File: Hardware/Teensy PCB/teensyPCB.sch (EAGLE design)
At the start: 14 parts, among them U2 USD-SOCKETNEW

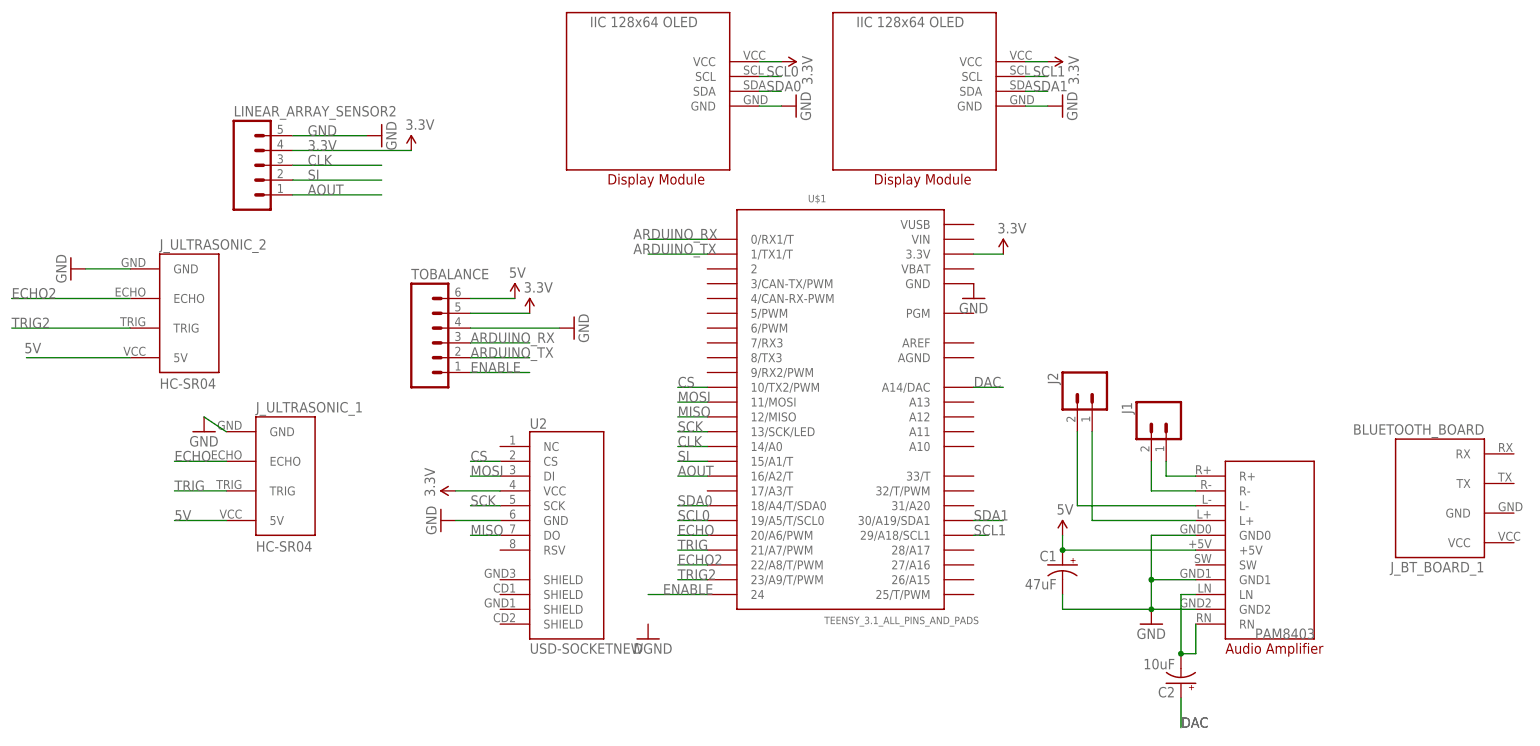
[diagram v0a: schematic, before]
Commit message: pcb update
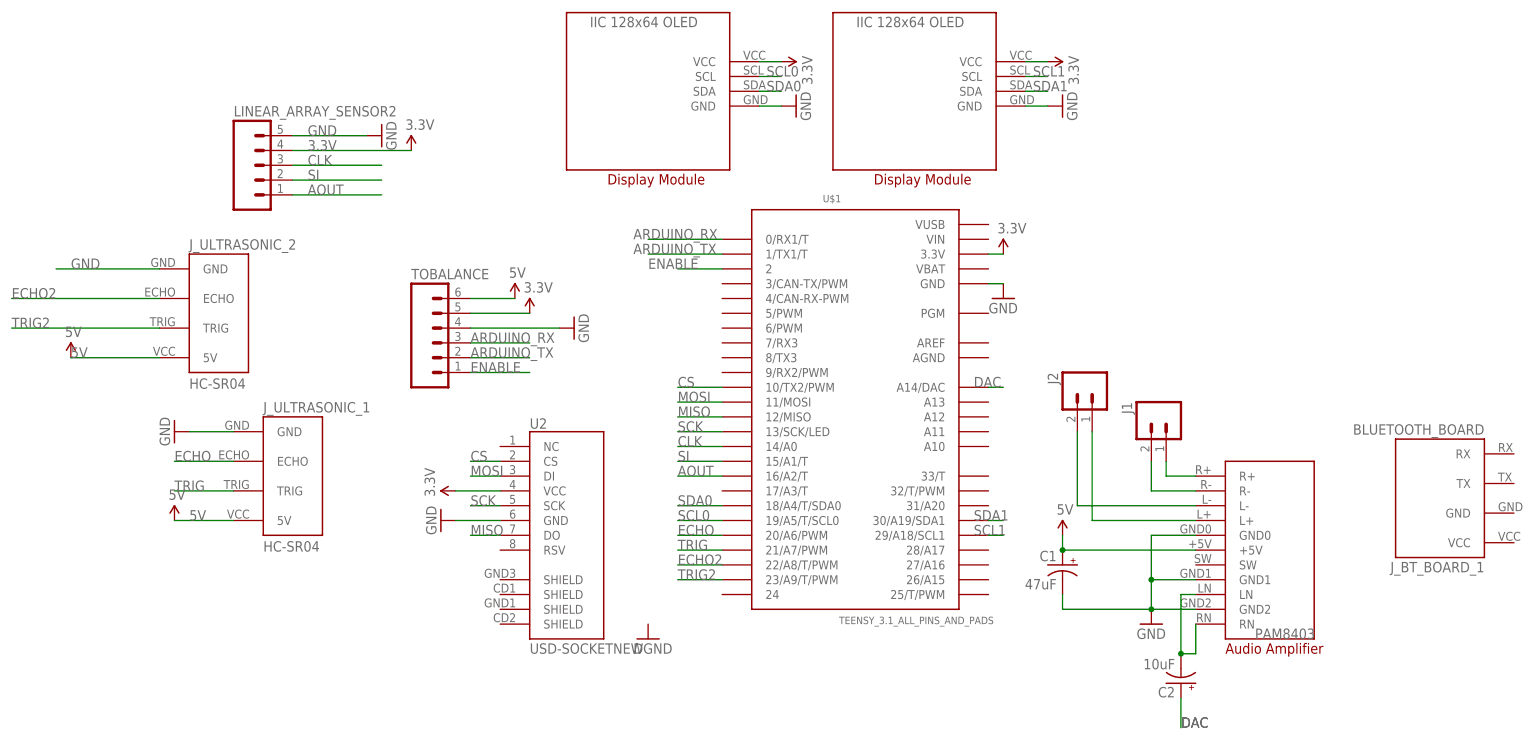
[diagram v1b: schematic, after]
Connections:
- net ENABLE: now also U$1.2; no longer U$1.24
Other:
- moved on the sheet: J_ULTRASONIC_1, J_ULTRASONIC_2, U$1
